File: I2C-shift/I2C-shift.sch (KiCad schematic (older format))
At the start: 11 parts, among them J1 I2C/5V, J2 I2C/5V, J3 I2C/12V, U1 TCA9548AMRGER, U2 P82B96, U3 AMS1117-5.0

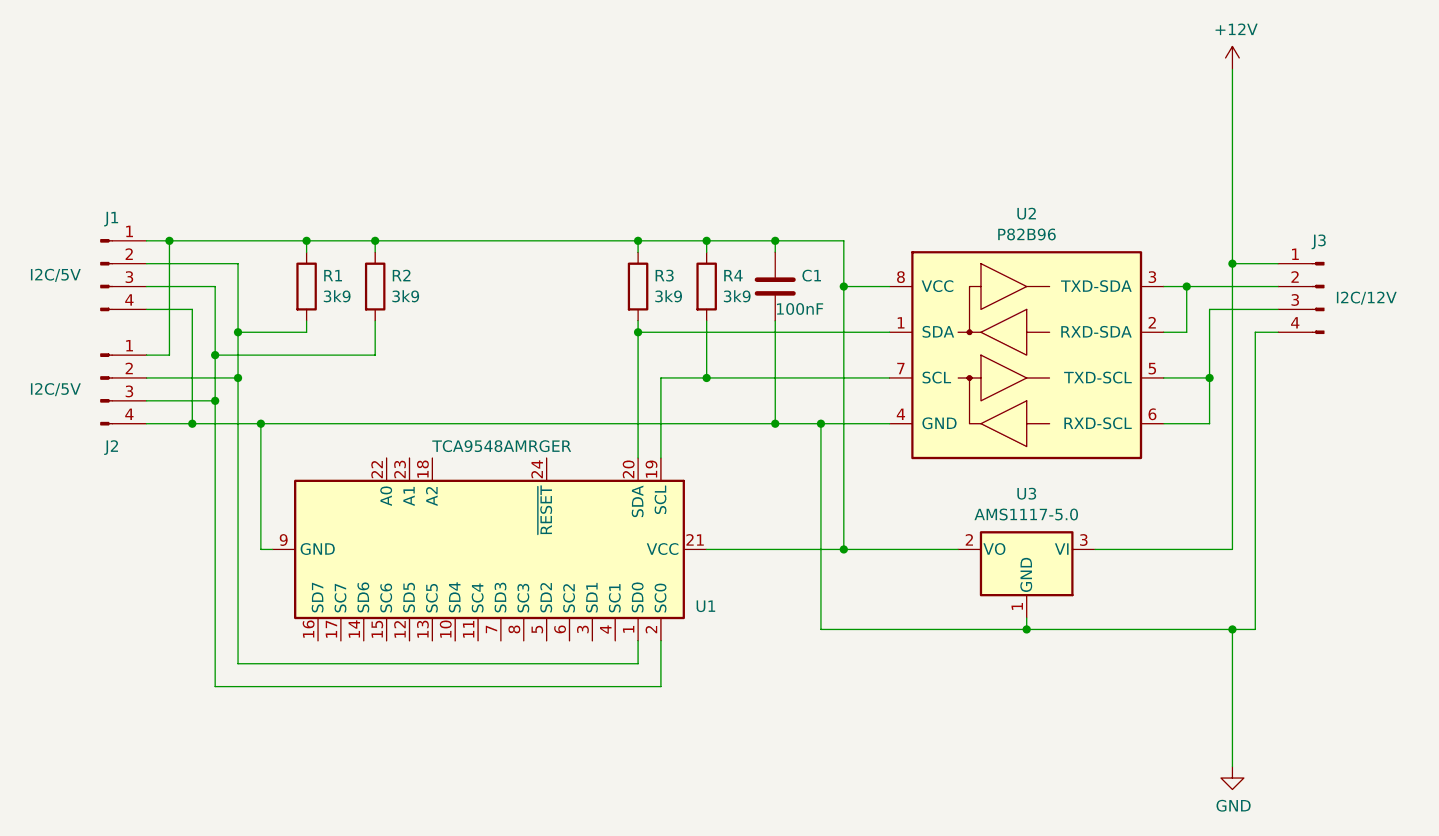
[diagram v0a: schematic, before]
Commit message: update electronic circuit
Signed-off-by: Samira-I2C <franz.siegele@gmx.net>
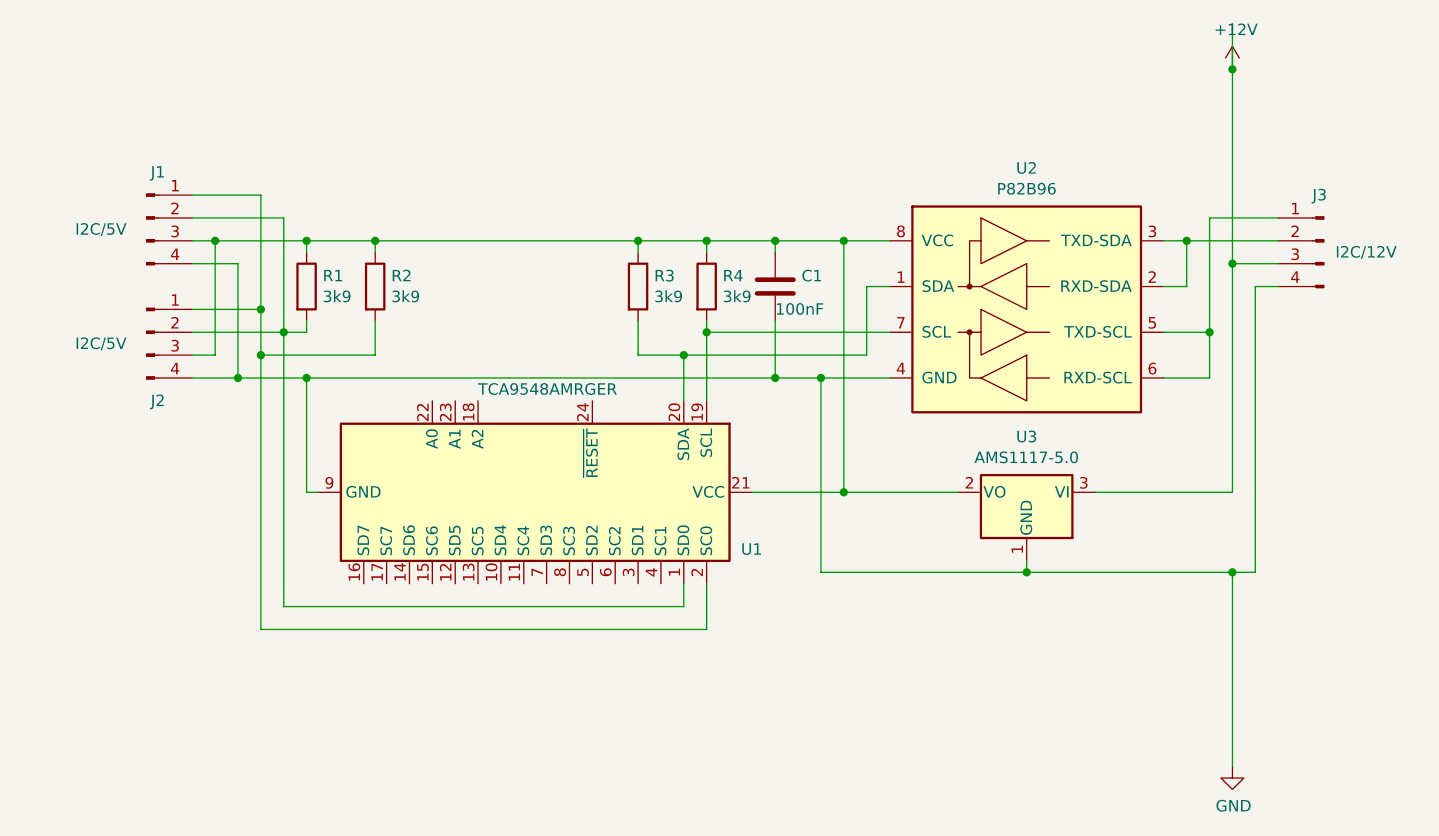
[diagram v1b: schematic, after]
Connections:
- net +12V: now also J3.3 (Pin_3); no longer J3.1 (Pin_1)
- net at U2.5 (TXD-SCL), U2.6 (RXD-SCL): now also J3.1 (Pin_1); no longer J3.3 (Pin_3)
- net at C1.1, R1.1, R2.1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: now also J1.3 (Pin_3), J2.3 (Pin_3); no longer J1.1 (Pin_1), J2.1 (Pin_1)
- net at R2.2, U1.2 (SC0): now also J1.1 (Pin_1), J2.1 (Pin_1); no longer J1.3 (Pin_3), J2.3 (Pin_3)
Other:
- moved on the sheet: J1, J2, J3, U1, U2, U3
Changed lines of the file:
@@
 L Interface_Expansion:P82B96 U2
 U 1 1 5EDB8D09
-P 6950 3350
-F 0 "U2" H 6950 3967 50  0000 C CNN
-F 1 "P82B96" H 6950 3876 50  0000 C CNN
-F 2 "" H 6950 3350 50  0001 C CNN
-F 3 "http://www.nxp.com/documents/data_sheet/P82B96.pdf" H 6950 3350 50  0001 C CNN
-	1    6950 3350
+P 6950 3150
+F 0 "U2" H 6950 3767 50  0000 C CNN
+F 1 "P82B96" H 6950 3676 50  0000 C CNN
+F 2 "" H 6950 3150 50  0001 C CNN
+F 3 "http://www.nxp.com/documents/data_sheet/P82B96.pdf" H 6950 3150 50  0001 C CNN
+	1    6950 3150
 	1    0    0    -1
 $EndComp
@@
 L Interface_Expansion:TCA9548AMRGER U1
 U 1 1 5EDBCB16
-P 4650 4200
-F 0 "U1" V 4900 5050 50  0000 L CNN
-F 1 "TCA9548AMRGER" V 4200 3900 50  0000 L CNN
-F 2 "Package_DFN_QFN:Texas_RGE0024C_EP2.1x2.1mm" H 4650 3200 50  0001 C CNN
-F 3 "http://www.ti.com/lit/ds/symlink/tca9548a.pdf" H 4700 4450 50  0001 C CNN
-	1    4650 4200
+P 4850 3950
+F 0 "U1" V 5100 4800 50  0000 L CNN
+F 1 "TCA9548AMRGER" V 4400 3650 50  0000 L CNN
+F 2 "Package_DFN_QFN:Texas_RGE0024C_EP2.1x2.1mm" H 4850 2950 50  0001 C CNN
+F 3 "http://www.ti.com/lit/ds/symlink/tca9548a.pdf" H 4900 4200 50  0001 C CNN
+	1    4850 3950
 	0    1    1    0
 $EndComp
 Wire Wire Line
-	5350 3450 5550 3450
-Wire Wire Line
-	5350 3450 5350 3800
-Wire Wire Line
-	5250 3250 5250 3800
-Wire Wire Line
-	3600 3650 3600 4200
-Wire Wire Line
-	3600 4200 3650 4200
+	3800 3950 3850 3950
 $Comp
 L Device:R R3
@@
 $EndComp
 Wire Wire Line
-	6150 3050 6350 3050
-Wire Wire Line
-	5250 3200 5250 3250
-Connection ~ 5250 3250
-Wire Wire Line
-	5550 3200 5550 3450
-Connection ~ 5550 3450
+	6150 2850 6350 2850
 Wire Wire Line
 	5250 2900 5250 2850
@@
 Wire Wire Line
 	5550 2850 5550 2900
-Wire Wire Line
-	6150 2850 6150 3050
 Connection ~ 5550 2850
-Connection ~ 6150 3050
 $Comp
 L Connector:Conn_01x04_Male J3
 U 1 1 5EDC76AF
-P 8250 3050
-F 0 "J3" H 8300 3250 50  0000 R CNN
-F 1 "I2C/12V" H 8200 3000 50  0000 R CNN
-F 2 "" H 8250 3050 50  0001 C CNN
-F 3 "~" H 8250 3050 50  0001 C CNN
-	1    8250 3050
+P 8250 2850
+F 0 "J3" H 8300 3050 50  0000 R CNN
+F 1 "I2C/12V" H 8200 2800 50  0000 R CNN
+F 2 "" H 8250 2850 50  0001 C CNN
+F 3 "~" H 8250 2850 50  0001 C CNN
+	1    8250 2850
 	-1   0    0    -1
 $EndComp
@@
 L Connector:Conn_01x04_Male J1
 U 1 1 5EDC8EDD
-P 2900 2950
-F 0 "J1" H 2950 3150 50  0000 C CNN
-F 1 "I2C/5V" H 2700 2900 50  0000 C CNN
-F 2 "" H 2900 2950 50  0001 C CNN
-F 3 "~" H 2900 2950 50  0001 C CNN
-	1    2900 2950
+P 3100 2750
+F 0 "J1" H 3150 2950 50  0000 C CNN
+F 1 "I2C/5V" H 2900 2700 50  0000 C CNN
+F 2 "" H 3100 2750 50  0001 C CNN
+F 3 "~" H 3100 2750 50  0001 C CNN
+	1    3100 2750
 	1    0    0    -1
 $EndComp
@@
 L Connector:Conn_01x04_Male J2
 U 1 1 5EDC98C1
-P 2900 3450
-F 0 "J2" H 2950 3150 50  0000 C CNN
-F 1 "I2C/5V" H 2700 3400 50  0000 C CNN
-F 2 "" H 2900 3450 50  0001 C CNN
-F 3 "~" H 2900 3450 50  0001 C CNN
-	1    2900 3450
+P 3100 3250
+F 0 "J2" H 3150 2950 50  0000 C CNN
+F 1 "I2C/5V" H 2900 3200 50  0000 C CNN
+F 2 "" H 3100 3250 50  0001 C CNN
+F 3 "~" H 3100 3250 50  0001 C CNN
+	1    3100 3250
 	1    0    0    -1
 $EndComp
@@
 Connection ~ 5250 2850
 Wire Wire Line
-	3200 2850 3200 3350
-Connection ~ 3200 2850
-Wire Wire Line
-	3200 2850 3100 2850
-Wire Wire Line
-	3100 3350 3200 3350
-Wire Wire Line
-	3100 3650 3300 3650
-Connection ~ 3600 3650
-Wire Wire Line
-	3100 3150 3300 3150
-Wire Wire Line
-	3300 3150 3300 3650
-Connection ~ 3300 3650
-Wire Wire Line
-	3300 3650 3600 3650
-Wire Wire Line
-	3100 2950 3500 2950
-Wire Wire Line
-	3500 2950 3500 3250
-Wire Wire Line
-	3500 4700 5250 4700
-Wire Wire Line
-	5250 4700 5250 4600
-Wire Wire Line
-	3100 3050 3400 3050
-Wire Wire Line
-	3400 3050 3400 3350
-Wire Wire Line
-	3400 4800 5350 4800
-Wire Wire Line
-	5350 4800 5350 4600
-Wire Wire Line
-	3100 3450 3500 3450
-Connection ~ 3500 3450
-Wire Wire Line
-	3500 3450 3500 4700
-Wire Wire Line
-	3100 3550 3400 3550
-Connection ~ 3400 3550
-Wire Wire Line
-	3400 3550 3400 4800
-Wire Wire Line
-	7550 3050 7650 3050
-Wire Wire Line
-	7650 3050 7650 3250
-Wire Wire Line
-	7650 3250 7550 3250
-Wire Wire Line
-	8050 3050 7650 3050
-Connection ~ 7650 3050
-Wire Wire Line
-	8050 3150 7750 3150
-Wire Wire Line
-	7750 3150 7750 3450
-Wire Wire Line
-	7750 3650 7750 3450
-Connection ~ 7750 3450
+	3700 4450 5450 4450
+Wire Wire Line
+	5450 4450 5450 4350
+Wire Wire Line
+	3600 4550 5550 4550
+Wire Wire Line
+	5550 4550 5550 4350
+Wire Wire Line
+	7550 2850 7650 2850
+Wire Wire Line
+	7650 2850 7650 3050
+Wire Wire Line
+	7650 3050 7550 3050
+Wire Wire Line
+	8050 2850 7650 2850
+Connection ~ 7650 2850
+Wire Wire Line
+	7750 3450 7750 3250
+Connection ~ 7750 3250
+Wire Wire Line
+	7550 3250 7750 3250
 Wire Wire Line
 	7550 3450 7750 3450
-Wire Wire Line
-	7550 3650 7750 3650
 $Comp
 L Regulator_Linear:AMS1117-5.0 U3
 U 1 1 5EDD656E
-P 6950 4200
-F 0 "U3" H 6950 4442 50  0000 C CNN
-F 1 "AMS1117-5.0" H 6950 4351 50  0000 C CNN
-F 2 "Package_TO_SOT_SMD:SOT-223-3_TabPin2" H 6950 4400 50  0001 C CNN
-F 3 "http://www.advanced-monolithic.com/pdf/ds1117.pdf" H 7050 3950 50  0001 C CNN
-	1    6950 4200
+P 6950 3950
+F 0 "U3" H 6950 4192 50  0000 C CNN
+F 1 "AMS1117-5.0" H 6950 4101 50  0000 C CNN
+F 2 "Package_TO_SOT_SMD:SOT-223-3_TabPin2" H 6950 4150 50  0001 C CNN
+F 3 "http://www.advanced-monolithic.com/pdf/ds1117.pdf" H 7050 3700 50  0001 C CNN
+	1    6950 3950
 	-1   0    0    -1
 $EndComp
 Wire Wire Line
-	6650 4200 6150 4200
-Wire Wire Line
-	7250 4200 7850 4200
-Wire Wire Line
-	7850 4200 7850 2950
-Wire Wire Line
-	7850 2950 8050 2950
-Wire Wire Line
-	6950 4500 6950 4550
-Wire Wire Line
-	6950 4550 7850 4550
-Wire Wire Line
-	7950 4550 7950 3250
-Wire Wire Line
-	7950 3250 8050 3250
-Connection ~ 6950 4550
+	7250 3950 7850 3950
+Wire Wire Line
+	6950 4250 6950 4300
+Wire Wire Line
+	6950 4300 7850 4300
+Wire Wire Line
+	7950 3050 8050 3050
+Connection ~ 6950 4300
 $Comp
 L Device:C C1
@@
 $EndComp
 Wire Wire Line
-	6150 3050 6150 4200
-Wire Wire Line
 	5550 2850 5850 2850
 $Comp
@@
 	1    0    0    -1
 $EndComp
-Wire Wire Line
-	7850 5150 7850 4550
-Connection ~ 7850 4550
-Wire Wire Line
-	7850 4550 7950 4550
+Connection ~ 7850 4300
+Wire Wire Line
+	7850 4300 7950 4300
 $Comp
 L power:+12V #PWR01
@@
 	1    0    0    -1
 $EndComp
-Wire Wire Line
-	7850 2100 7850 2950
-Connection ~ 7850 2950
 $Comp
 L Device:R R1
@@
 Connection ~ 3800 2850
 Wire Wire Line
-	3800 2850 3200 2850
-Wire Wire Line
-	3800 3200 3800 3250
-Wire Wire Line
-	3800 3250 3500 3250
-Connection ~ 3500 3250
-Wire Wire Line
-	3500 3250 3500 3450
-Wire Wire Line
-	4100 3200 4100 3350
-Wire Wire Line
-	4100 3350 3400 3350
-Connection ~ 3400 3350
-Wire Wire Line
-	3400 3350 3400 3550
-Wire Wire Line
 	5850 2900 5850 2850
 Connection ~ 5850 2850
 Wire Wire Line
-	5850 3200 5850 3650
-Connection ~ 5850 3650
-Wire Wire Line
-	3600 3650 5850 3650
+	5850 3200 5850 3450
 Wire Wire Line
 	5850 2850 6150 2850
 Wire Wire Line
-	5250 3250 6350 3250
-Wire Wire Line
-	5550 3450 6350 3450
-Wire Wire Line
-	5850 3650 6050 3650
-Wire Wire Line
-	6050 3650 6050 4550
-Connection ~ 6050 3650
-Wire Wire Line
-	6050 4550 6950 4550
-Wire Wire Line
-	6050 3650 6350 3650
-Wire Wire Line
-	5550 4200 6150 4200
-Connection ~ 6150 4200
+	6050 4300 6950 4300
+Wire Wire Line
+	6050 3450 6350 3450
+Wire Wire Line
+	5750 3950 6150 3950
+Connection ~ 6150 3950
+Wire Wire Line
+	7850 1900 7850 2100
+Wire Wire Line
+	8050 2950 7850 2950
+Connection ~ 7850 2950
+Wire Wire Line
+	7750 2750 8050 2750
+Wire Wire Line
+	7750 2750 7750 3250
+Connection ~ 6150 2850
+Connection ~ 7850 2100
+Wire Wire Line
+	5250 3200 5250 3350
+Wire Wire Line
+	5550 3200 5550 3250
+Connection ~ 5550 3250
+Wire Wire Line
+	5550 3250 6350 3250
+Wire Wire Line
+	6350 3050 6250 3050
+Wire Wire Line
+	6250 3050 6250 3350
+Wire Wire Line
+	6250 3350 5450 3350
+Connection ~ 5450 3350
+Wire Wire Line
+	5450 3350 5250 3350
+Wire Wire Line
+	6050 3450 5850 3450
+Wire Wire Line
+	6150 3950 6650 3950
+Connection ~ 6050 3450
+Connection ~ 5850 3450
+Wire Wire Line
+	5850 3450 3800 3450
+Wire Wire Line
+	3800 3200 3800 3250
+Wire Wire Line
+	3800 3450 3500 3450
+Connection ~ 3800 3450
+Wire Wire Line
+	3600 2650 3300 2650
+Connection ~ 3600 3150
+Wire Wire Line
+	3600 3150 3600 3350
+Wire Wire Line
+	3600 3350 4100 3350
+Wire Wire Line
+	4100 3350 4100 3200
+Connection ~ 3600 3350
+Wire Wire Line
+	3700 4450 3700 3250
+Wire Wire Line
+	3700 2750 3300 2750
+Connection ~ 3700 3250
+Wire Wire Line
+	3700 3250 3800 3250
+Wire Wire Line
+	3500 3450 3500 2950
+Connection ~ 3500 3450
+Wire Wire Line
+	3400 2850 3400 3350
+Connection ~ 3400 2850
+Wire Wire Line
+	3400 2850 3800 2850
+Wire Wire Line
+	3300 3150 3600 3150
+Wire Wire Line
+	3300 3250 3700 3250
+Wire Wire Line
+	3300 3350 3400 3350
+Wire Wire Line
+	3300 3450 3500 3450
+Wire Wire Line
+	3300 2850 3400 2850
+Wire Wire Line
+	3300 2950 3500 2950
+Wire Wire Line
+	7950 3050 7950 4300
+Wire Wire Line
+	7850 2950 7850 3950
+Wire Wire Line
+	6150 2850 6150 3950
+Wire Wire Line
+	5550 3250 5550 3550
+Wire Wire Line
+	5450 3350 5450 3550
+Wire Wire Line
+	6050 3450 6050 4300
+Wire Wire Line
+	3800 3450 3800 3950
+Wire Wire Line
+	3600 3350 3600 4550
+Wire Wire Line
+	7850 2100 7850 2950
+Wire Wire Line
+	3600 2650 3600 3150
+Wire Wire Line
+	3700 2750 3700 3250
+Wire Wire Line
+	7850 4300 7850 5150
 $EndSCHEMATC
